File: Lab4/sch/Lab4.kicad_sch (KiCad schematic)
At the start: 3 parts, among them SW1 SW_Push, U1 2478, U2 Pico

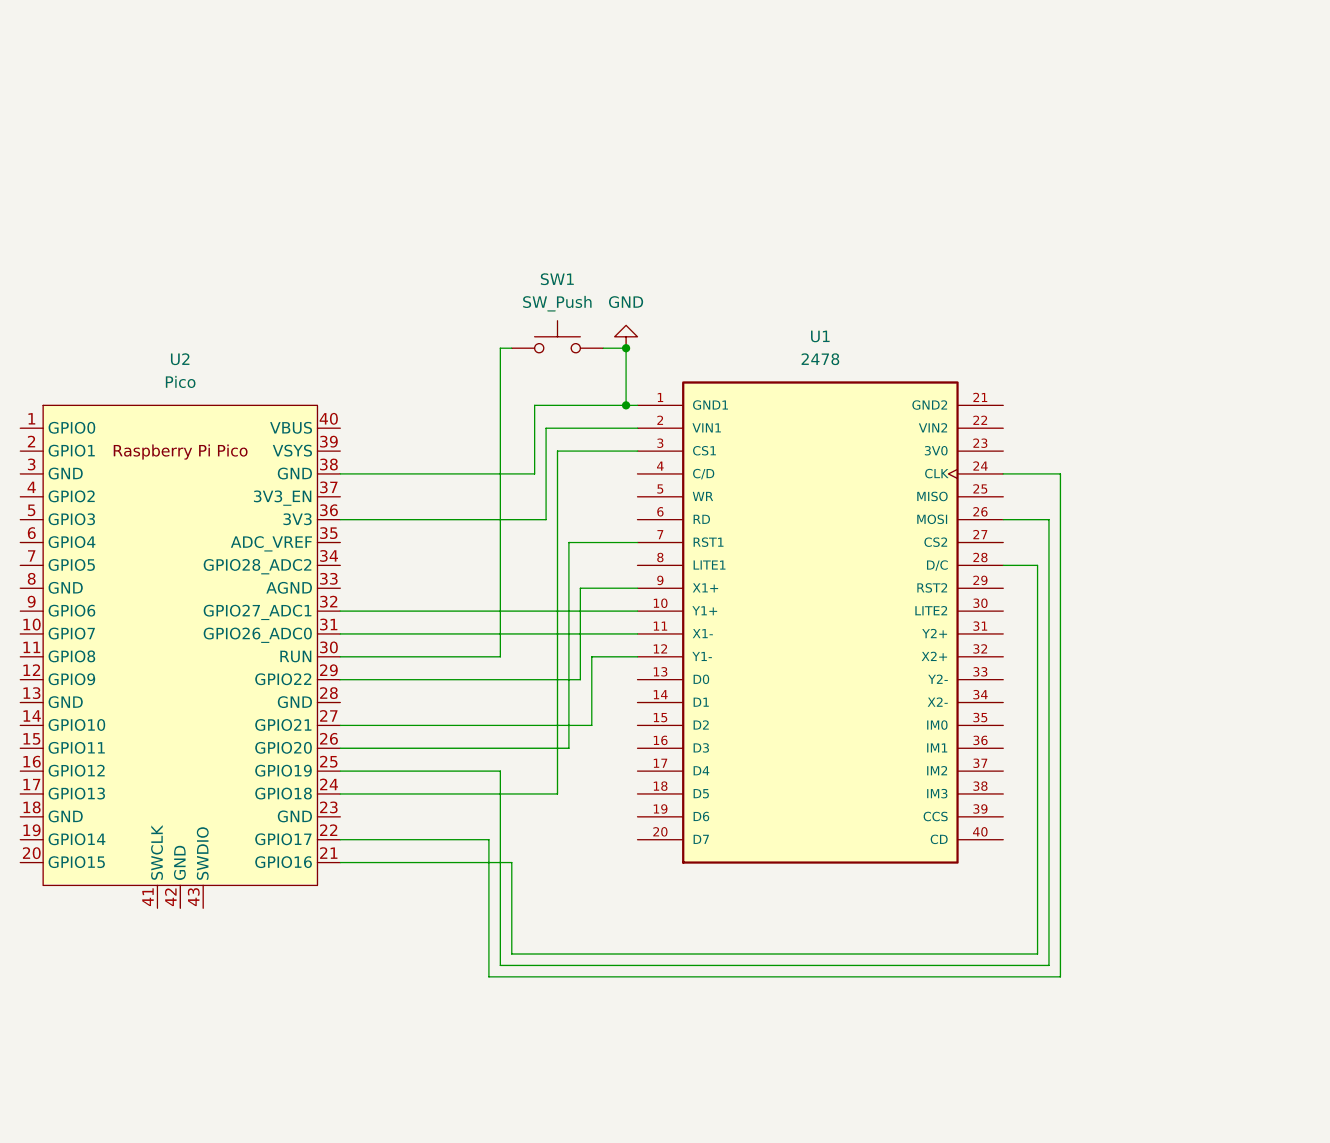
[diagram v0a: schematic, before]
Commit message: Final Version
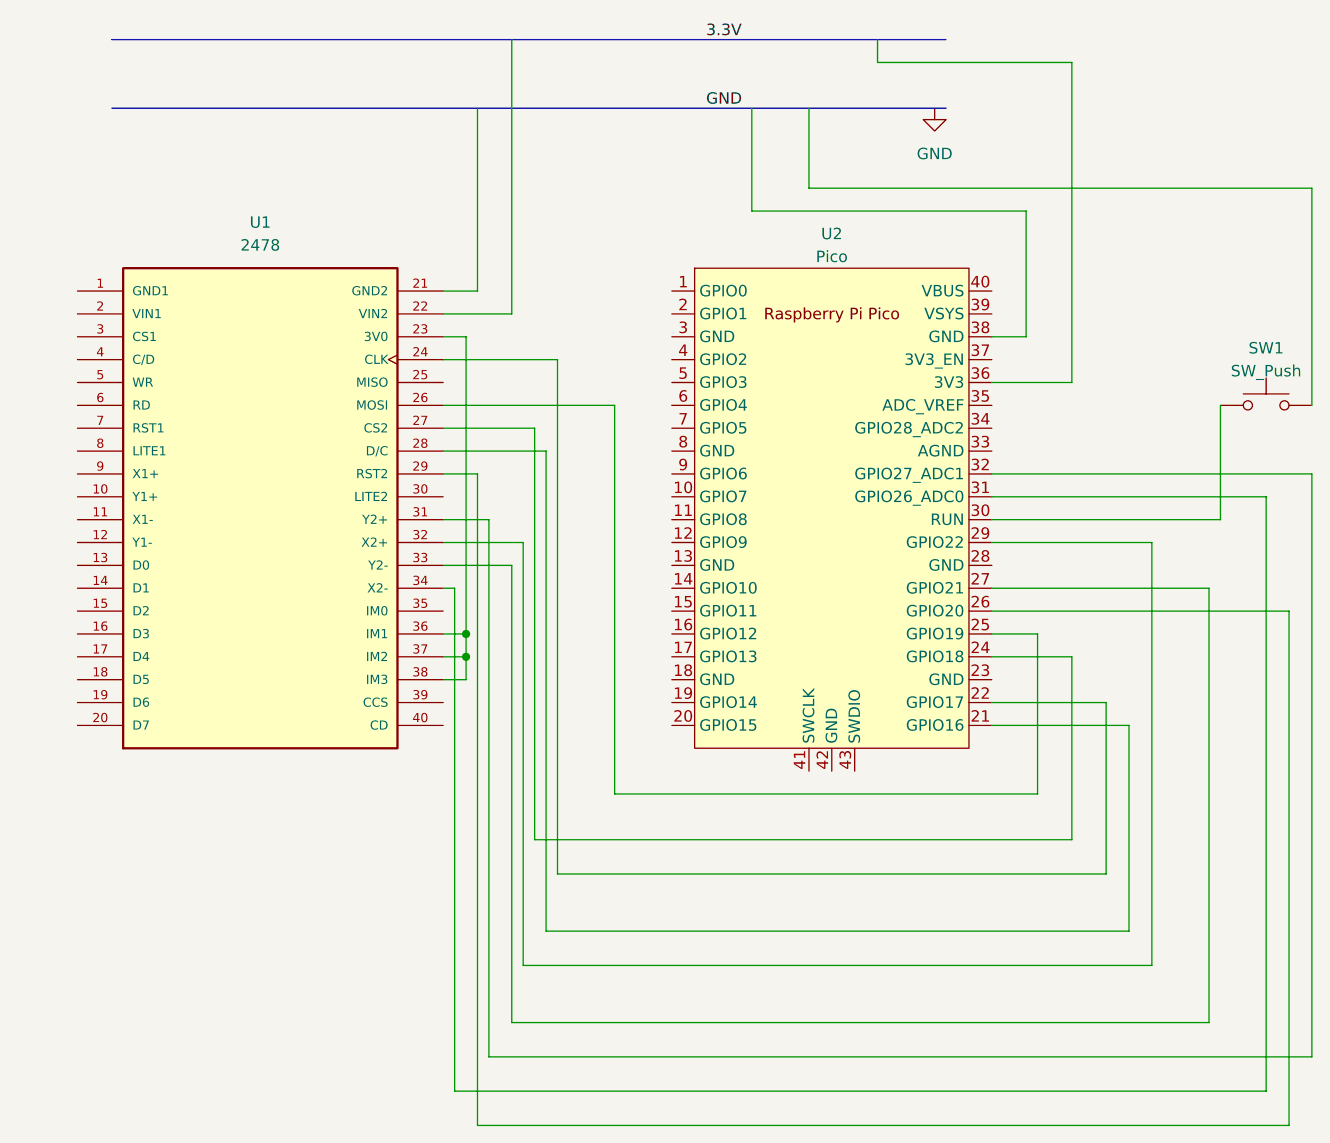
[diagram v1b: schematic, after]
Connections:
- net GND: no longer SW1.2, U1.1 (GND1), U2.38 (GND)
- net at U2.24 (GPIO18): now also U1.27 (CS2); no longer U1.3 (CS1)
- net at U2.26 (GPIO20): now also U1.29 (RST2); no longer U1.7 (RST1)
- net at U1.12 (Y1-): no longer U2.27 (GPIO21)
- net at U2.29 (GPIO22): now also U1.32 (X2+); no longer U1.9 (X1+)
- net at U1.11 (X1-): no longer U2.31 (GPIO26_ADC0)
- net at U1.10 (Y1+): no longer U2.32 (GPIO27_ADC1)
- net at U1.2 (VIN1): no longer U2.36 (3V3)
- net at U1.23 (3V0): now also U1.36 (IM1), U1.37 (IM2), U1.38 (IM3)
- net at U1.31 (Y2+): now also U2.32 (GPIO27_ADC1)
- net at U1.33 (Y2-): now also U2.27 (GPIO21)
- net at U1.34 (X2-): now also U2.31 (GPIO26_ADC0)
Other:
- company: Lafayette College -> Lafayette College 
